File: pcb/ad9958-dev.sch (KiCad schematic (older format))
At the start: 88 parts, among them J1 INTERFACE, J2 5V, J3 OUT1, J4 OUT0, U1 AZ1117CH-1.8TRG1, U2 AD9958, U3 LMH6714MF, U4 LMH6714MF, X1 25 MHz

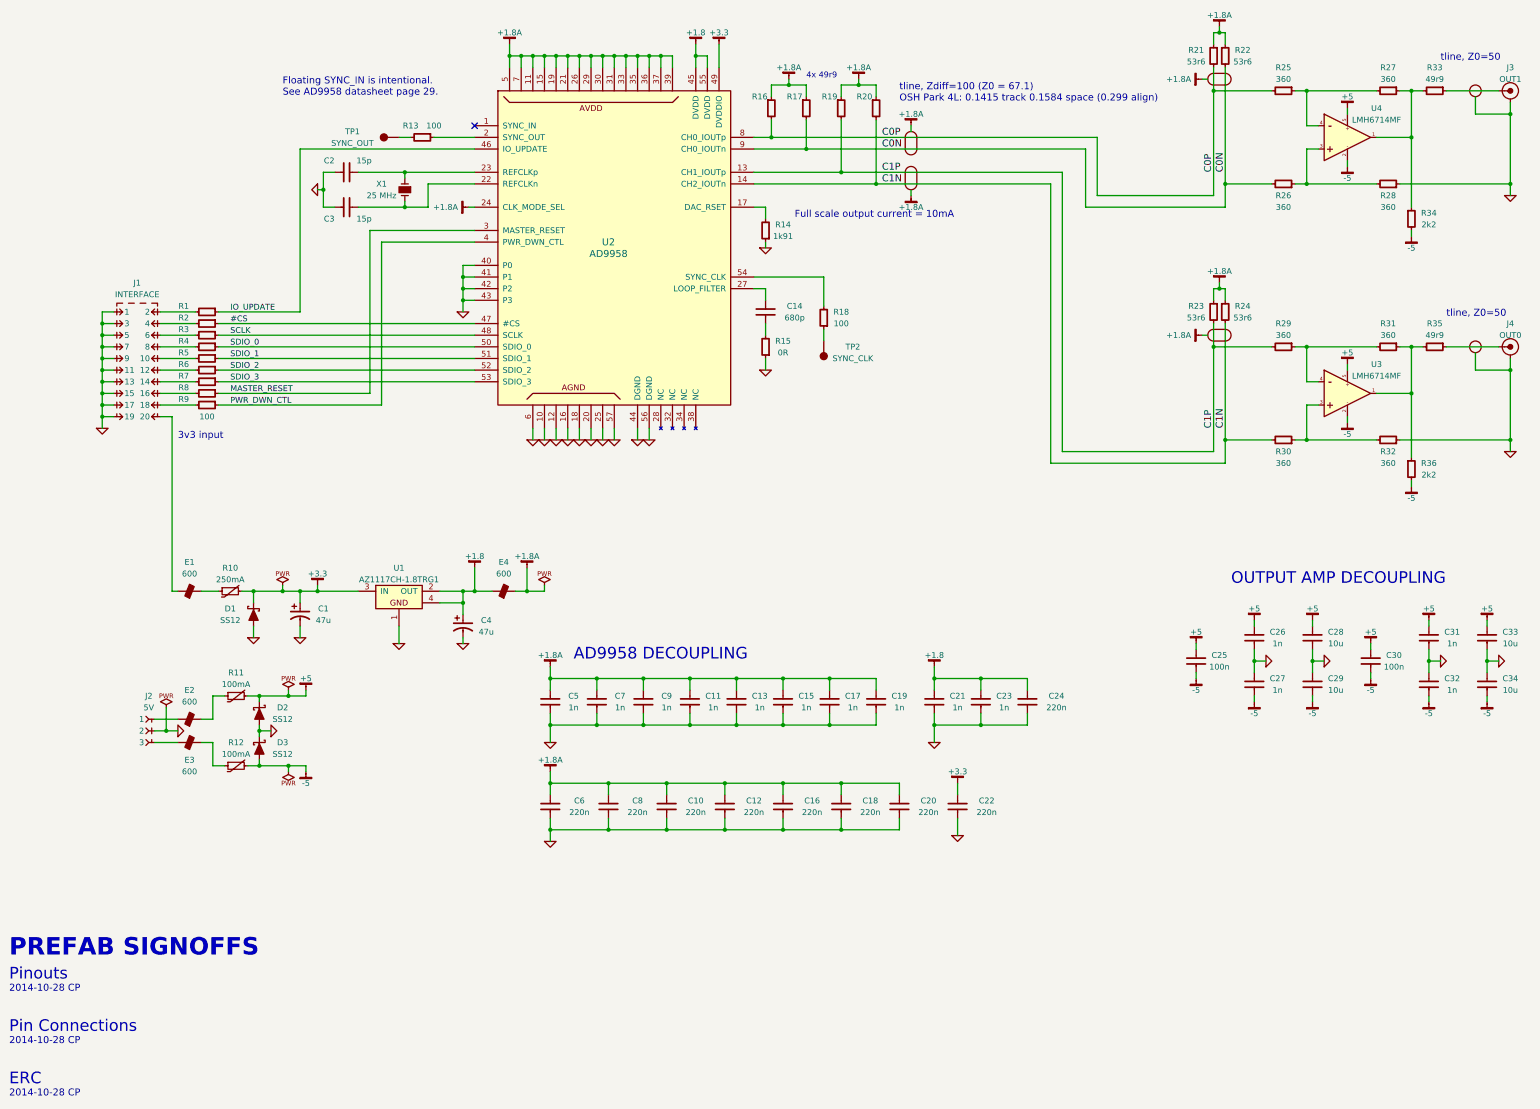
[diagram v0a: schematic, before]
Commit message: Updated schematic render
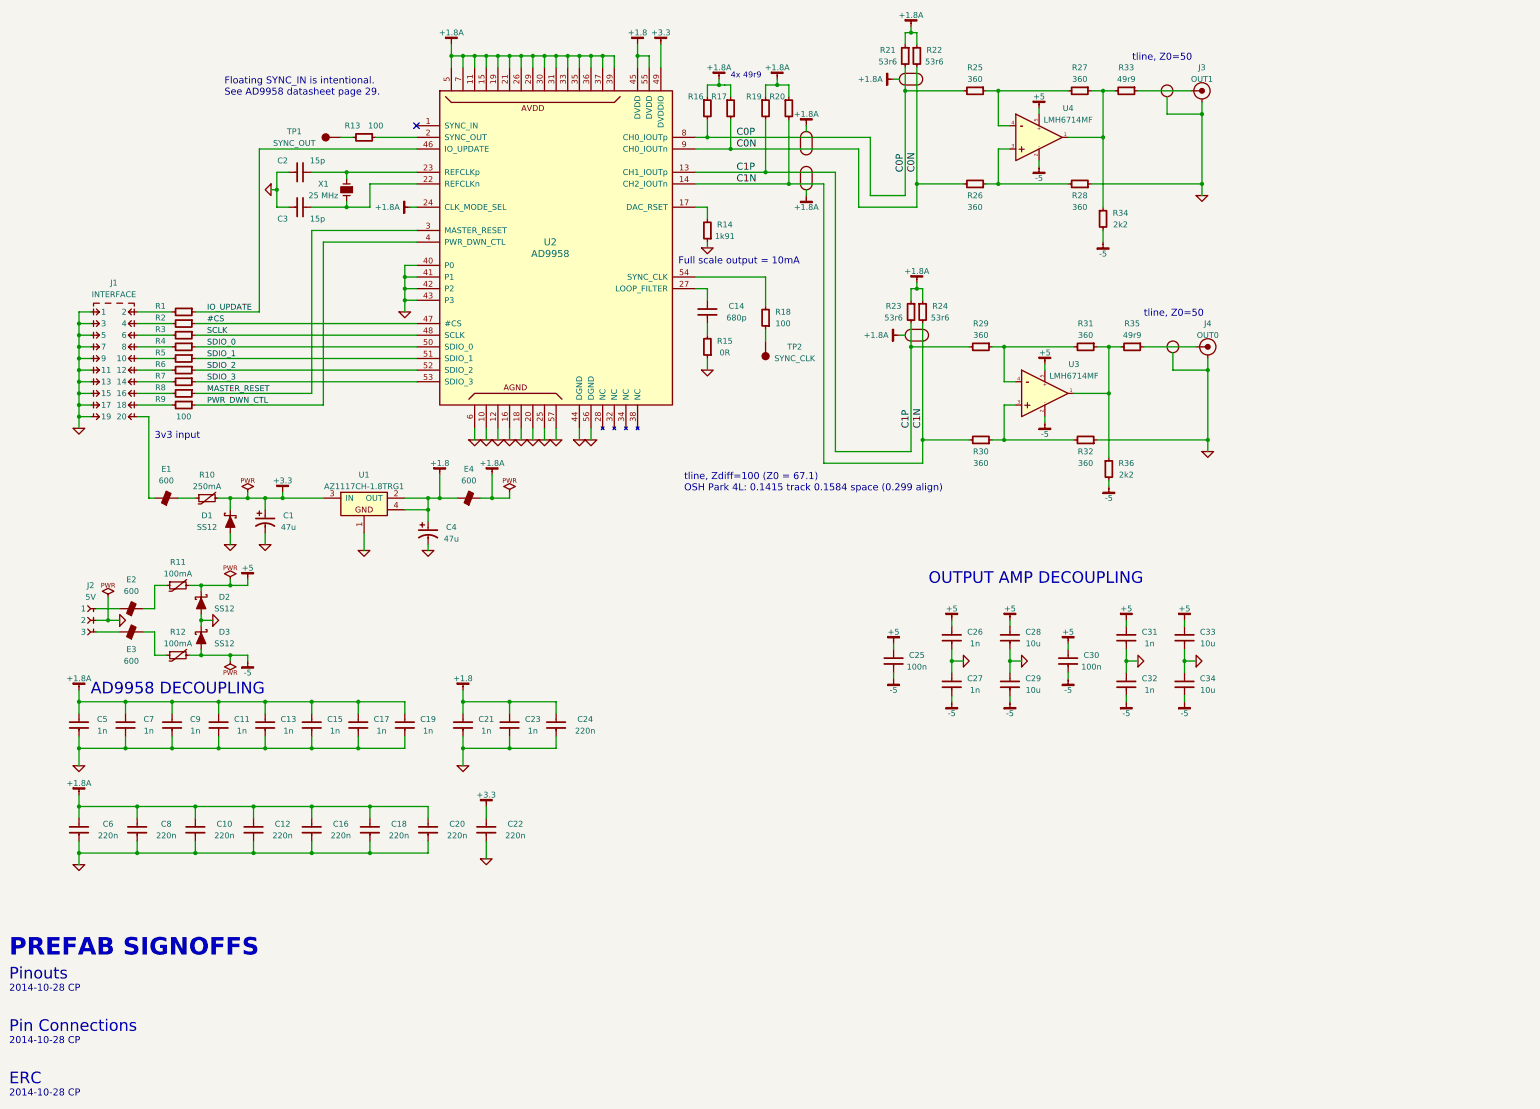
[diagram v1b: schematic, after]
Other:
- note added: "Full scale output = 10mA"
- note removed: "Full scale output current = 10mA"
- moved on the sheet: C1, C10, C11, C12, C13, C14, C15, C16, C17, C18, C19, C2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
